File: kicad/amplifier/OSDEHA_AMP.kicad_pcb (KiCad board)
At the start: 2 copper layers, 190.1 x 72.4 mm, 86 parts, among them J1 INPUT, J2 HEATERS DC, J3 PSU HV, J4 OUTPUT, J5 DHT FIL2, J6 DHT FIL1, Q1 DN2540N5-G, Q10 DN2540, Q2 DN2540N5-G, Q3 STF3LN80K5, Q4 STF3LN80K5, Q5 AOT1N60, Q6 IXTP3N100D2, Q7 AOT1N60, Q8 IXTP3N100D2, Q9 DN2540, SW1 SW_DPDT_x2, U1 6E5P, U2 6E5P, U3 801A, U4 801A

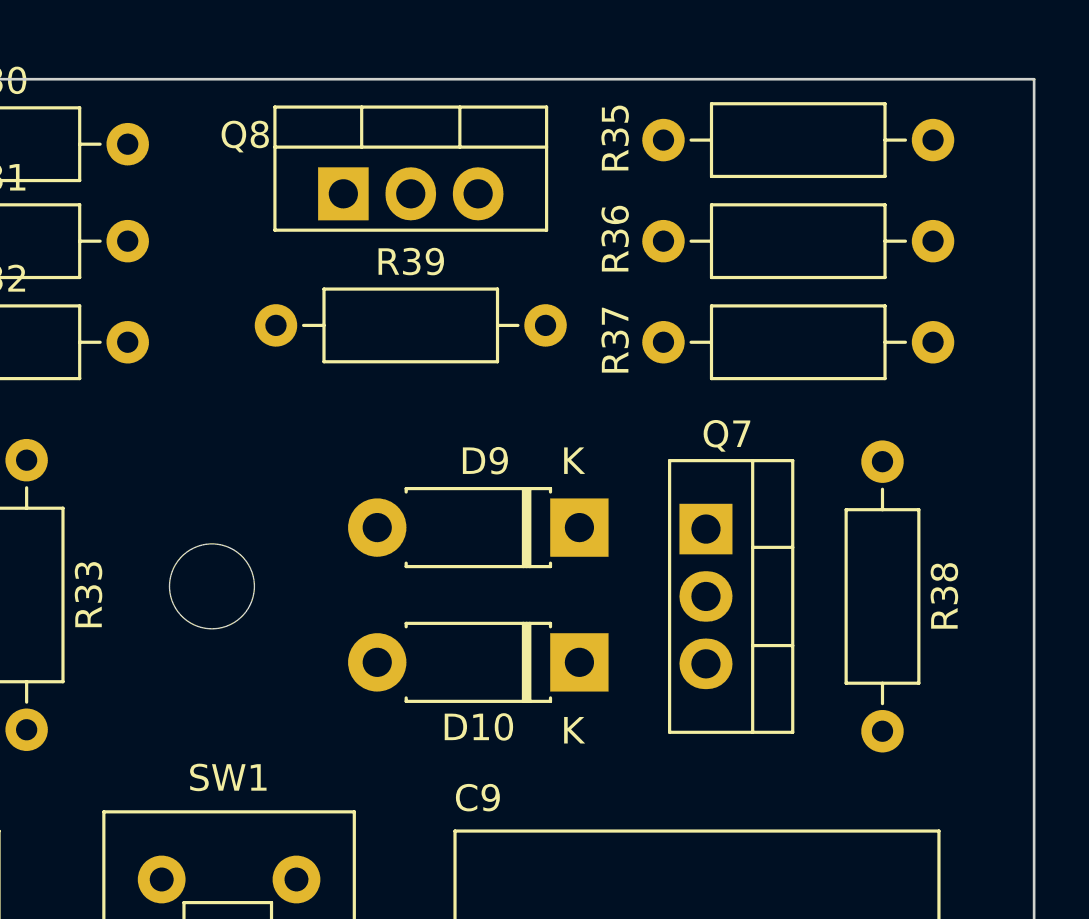
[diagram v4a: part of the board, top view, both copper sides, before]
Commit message: pcb
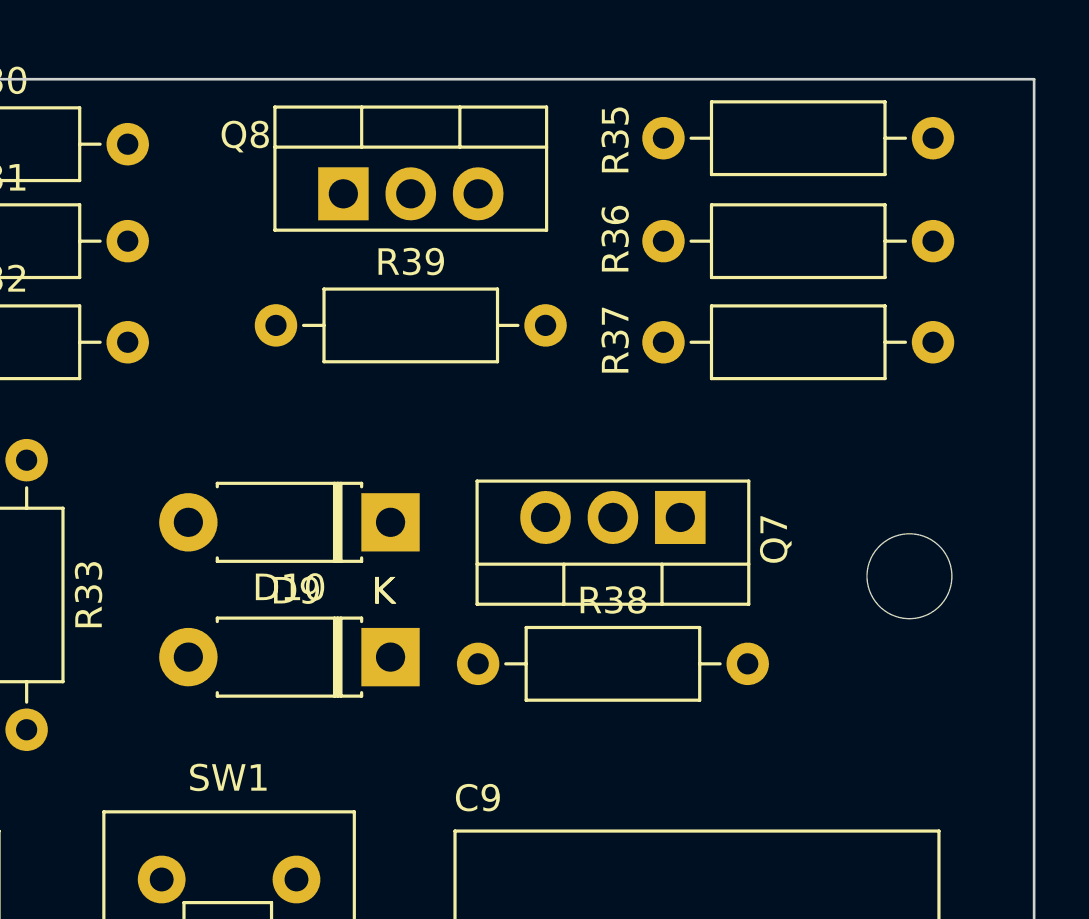
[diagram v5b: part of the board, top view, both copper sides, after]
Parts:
- moved H3 26.3 mm to (251.7, 67.6)
- moved R38 17.0 mm to (235.5, 70.9), turned to 0 degrees
- moved R35 10.2 mm to (252.6, 51.1), turned to 180 degrees
- moved D10 8.86 mm to (232.2, 65.5)
- moved D9 8.63 mm to (232.2, 70.6)
- moved Q7 1.06 mm to (243.1, 65.3), turned to 180 degrees
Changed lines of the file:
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@@
   )
   (footprint "Diode_THT:D_DO-41_SOD81_P7.62mm_Horizontal" (layer "F.Cu")
-    (at 239.275 70.81 180)
+    (at 232.156 65.532 180)
     (descr "Diode, DO-41_SOD81 series, Axial, Horizontal, pin pitch=7.62mm, , length*diameter=5.2*2.7mm^2, , http://www.diodes.com/_files/packages/DO-41%20(Plastic).pdf")
     (tags "Diode DO-41_SOD81 series Axial Horizontal pin pitch 7.62mm  length 5.2mm diameter 2.7mm")
@@
   )
   (footprint "MountingHole:MountingHole_3.2mm_M3" (layer "F.Cu")
-    (at 225.425 67.945)
+    (at 251.714 67.564)
     (descr "Mounting Hole 3.2mm, no annular, M3")
     (tags "mounting hole 3.2mm no annular m3")
@@
   )
   (footprint "Package_TO_SOT_THT:TO-220-3_Vertical" (layer "F.Cu")
-    (at 244.045 65.786 -90)
+    (at 243.078 65.349 180)
     (descr "TO-220-3, Vertical, RM 2.54mm, see https://www.vishay.com/docs/66542/to-220-1.pdf")
     (tags "TO-220-3 Vertical RM 2.54mm")
@@
     (property "ki_keywords" "N-Channel Depletion-Mode MOSFET")
     (attr through_hole)
-    (fp_text reference "Q7" (at -3.556 -0.811 -180) (layer "F.SilkS")
-        (effects (font (size 1 1) (thickness 0.15)))
-    )
-    (fp_text value "AOT1N60" (at 2.54 2.5 90) (layer "F.Fab")
-        (effects (font (size 1 1) (thickness 0.15)))
-    )
-    (fp_text user "${REFERENCE}" (at 2.54 -4.27 90) (layer "F.Fab")
+    (fp_text reference "Q7" (at -3.556 -0.811 90) (layer "F.SilkS")
+        (effects (font (size 1 1) (thickness 0.15)))
+    )
+    (fp_text value "AOT1N60" (at 2.54 2.5) (layer "F.Fab")
+        (effects (font (size 1 1) (thickness 0.15)))
+    )
+    (fp_text user "${REFERENCE}" (at 2.54 -4.27) (layer "F.Fab")
         (effects (font (size 1 1) (thickness 0.15)))
     )
@@
     (fp_line (start 7.54 1.25) (end 7.54 -3.15)
       (stroke (width 0.1) (type solid)) (layer "F.Fab"))
-    (pad "1" thru_hole rect (at 0 0 270) (size 1.905 2) (drill 1.1) (layers "*.Cu" "*.Mask")
+    (pad "1" thru_hole rect (at 0 0 180) (size 1.905 2) (drill 1.1) (layers "*.Cu" "*.Mask")
       (net 31 "Net-(D9-K)") (pinfunction "G") (pintype "input"))
-    (pad "2" thru_hole oval (at 2.54 0 270) (size 1.905 2) (drill 1.1) (layers "*.Cu" "*.Mask")
+    (pad "2" thru_hole oval (at 2.54 0 180) (size 1.905 2) (drill 1.1) (layers "*.Cu" "*.Mask")
       (net 35 "Net-(Q7-D)") (pinfunction "D") (pintype "passive"))
-    (pad "3" thru_hole oval (at 5.08 0 270) (size 1.905 2) (drill 1.1) (layers "*.Cu" "*.Mask")
+    (pad "3" thru_hole oval (at 5.08 0 180) (size 1.905 2) (drill 1.1) (layers "*.Cu" "*.Mask")
       (net 17 "/Dual_Gyrator/MU_OUT2") (pinfunction "S") (pintype "passive"))
     (model "${KICAD6_3DMODEL_DIR}/Package_TO_SOT_THT.3dshapes/TO-220-3_Vertical.wrl"
@@
   )
   (footprint "Resistor_THT:R_Axial_DIN0207_L6.3mm_D2.5mm_P10.16mm_Horizontal" (layer "F.Cu")
-    (at 250.698 63.246 -90)
+    (at 235.458 70.866)
     (descr "Resistor, Axial_DIN0207 series, Axial, Horizontal, pin pitch=10.16mm, 0.25W = 1/4W, length*diameter=6.3*2.5mm^2, http://cdn-reichelt.de/documents/datenblatt/B400/1_4W%23YAG.pdf")
     (tags "Resistor Axial_DIN0207 series Axial Horizontal pin pitch 10.16mm 0.25W = 1/4W length 6.3mm diameter 2.5mm")
@@
     (property "ki_keywords" "R res resistor")
     (attr through_hole)
-    (fp_text reference "R38" (at 5.08 -2.37 90) (layer "F.SilkS")
-        (effects (font (size 1 1) (thickness 0.15)))
-    )
-    (fp_text value "470" (at 5.08 2.37 90) (layer "F.Fab")
-        (effects (font (size 1 1) (thickness 0.15)))
-    )
-    (fp_text user "${REFERENCE}" (at 5.08 0 90) (layer "F.Fab")
+    (fp_text reference "R38" (at 5.08 -2.37) (layer "F.SilkS")
+        (effects (font (size 1 1) (thickness 0.15)))
+    )
+    (fp_text value "470" (at 5.08 2.37) (layer "F.Fab")
+        (effects (font (size 1 1) (thickness 0.15)))
+    )
+    (fp_text user "${REFERENCE}" (at 5.08 0) (layer "F.Fab")
         (effects (font (size 1 1) (thickness 0.15)))
     )
@@
     (fp_line (start 10.16 0) (end 8.23 0)
       (stroke (width 0.1) (type solid)) (layer "F.Fab"))
-    (pad "1" thru_hole circle (at 0 0 270) (size 1.6 1.6) (drill 0.8) (layers "*.Cu" "*.Mask")
+    (pad "1" thru_hole circle (at 0 0) (size 1.6 1.6) (drill 0.8) (layers "*.Cu" "*.Mask")
       (net 17 "/Dual_Gyrator/MU_OUT2") (pintype "passive"))
-    (pad "2" thru_hole oval (at 10.16 0 270) (size 1.6 1.6) (drill 0.8) (layers "*.Cu" "*.Mask")
+    (pad "2" thru_hole oval (at 10.16 0) (size 1.6 1.6) (drill 0.8) (layers "*.Cu" "*.Mask")
       (net 12 "/Dual_Gyrator/ANODE2") (pintype "passive"))
     (model "${KICAD6_3DMODEL_DIR}/Resistor_THT.3dshapes/R_Axial_DIN0207_L6.3mm_D2.5mm_P10.16mm_Horizontal.wrl"
@@
   )
   (footprint "Resistor_THT:R_Axial_DIN0207_L6.3mm_D2.5mm_P10.16mm_Horizontal" (layer "F.Cu")
-    (at 242.443 51.125)
+    (at 252.603 51.054 180)
     (descr "Resistor, Axial_DIN0207 series, Axial, Horizontal, pin pitch=10.16mm, 0.25W = 1/4W, length*diameter=6.3*2.5mm^2, http://cdn-reichelt.de/documents/datenblatt/B400/1_4W%23YAG.pdf")
     (tags "Resistor Axial_DIN0207 series Axial Horizontal pin pitch 10.16mm 0.25W = 1/4W length 6.3mm diameter 2.5mm")
@@
     (property "ki_keywords" "R res resistor")
     (attr through_hole)
-    (fp_text reference "R35" (at -1.785 -0.071 90) (layer "F.SilkS")
+    (fp_text reference "R35" (at 11.945 -0.071 90) (layer "F.SilkS")
         (effects (font (size 1 1) (thickness 0.15)))
     )
@@
     (fp_line (start 10.16 0) (end 8.23 0)
       (stroke (width 0.1) (type solid)) (layer "F.Fab"))
-    (pad "1" thru_hole circle (at 0 0) (size 1.6 1.6) (drill 0.8) (layers "*.Cu" "*.Mask")
+    (pad "1" thru_hole circle (at 0 0 180) (size 1.6 1.6) (drill 0.8) (layers "*.Cu" "*.Mask")
       (net 63 "Net-(R35-Pad1)") (pintype "passive"))
-    (pad "2" thru_hole oval (at 10.16 0) (size 1.6 1.6) (drill 0.8) (layers "*.Cu" "*.Mask")
+    (pad "2" thru_hole oval (at 10.16 0 180) (size 1.6 1.6) (drill 0.8) (layers "*.Cu" "*.Mask")
       (net 19 "GND") (pintype "passive"))
     (model "${KICAD6_3DMODEL_DIR}/Resistor_THT.3dshapes/R_Axial_DIN0207_L6.3mm_D2.5mm_P10.16mm_Horizontal.wrl"
@@
   )
   (footprint "Diode_THT:D_DO-41_SOD81_P7.62mm_Horizontal" (layer "F.Cu")
-    (at 239.275 65.73 180)
+    (at 232.156 70.612 180)
     (descr "Diode, DO-41_SOD81 series, Axial, Horizontal, pin pitch=7.62mm, , length*diameter=5.2*2.7mm^2, , http://www.diodes.com/_files/packages/DO-41%20(Plastic).pdf")
     (tags "Diode DO-41_SOD81 series Axial Horizontal pin pitch 7.62mm  length 5.2mm diameter 2.7mm")
